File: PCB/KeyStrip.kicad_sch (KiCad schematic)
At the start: 10 parts, among them J2 JST_08

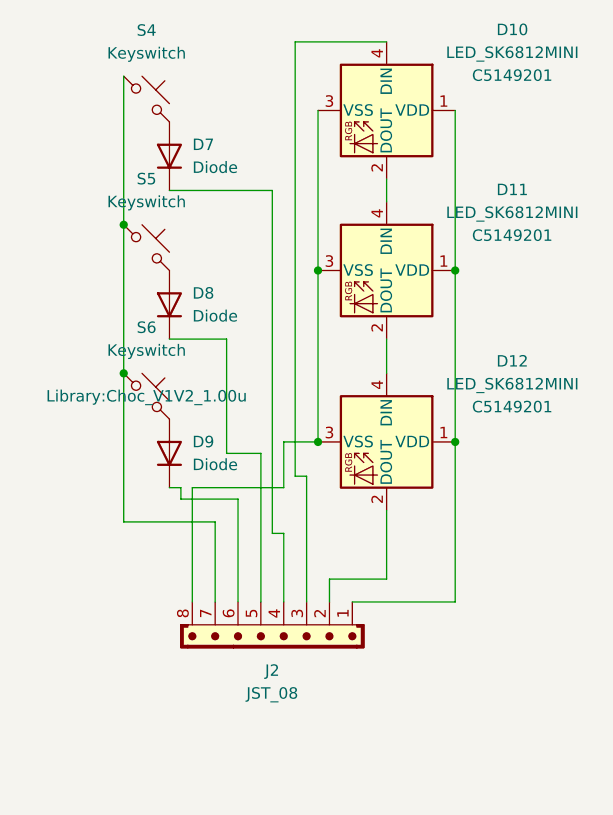
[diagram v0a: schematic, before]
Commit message: I just gotta add screw holes and solo variations now
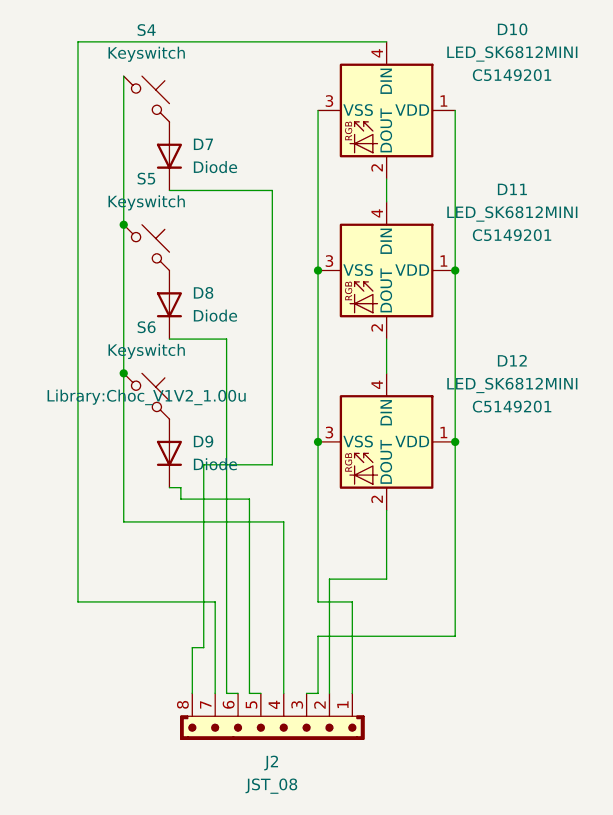
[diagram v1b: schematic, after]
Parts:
- J2: footprint Connector_JST:JST_EH_B8B-EH-A_1x08_P2.50mm_Vertical -> Library:JST_EH_B8B-EH-A_1x08_P2.50mm_Vertical
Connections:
- net at D7.1 (K): now also J2.8; no longer J2.4
- net at S4.1, S5.1, S6.1: now also J2.4; no longer J2.7
- net at D10.1 (VDD), D11.1 (VDD), D12.1 (VDD): now also J2.3; no longer J2.1
- net at D10.4 (DIN): now also J2.7; no longer J2.3
- net at J2.5: now also D9.1 (K); no longer D8.1 (K)
- net at J2.6: now also D8.1 (K); no longer D9.1 (K)
- net at D10.3 (VSS), D11.3 (VSS), D12.3 (VSS): now also J2.1; no longer J2.8
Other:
- moved on the sheet: J2
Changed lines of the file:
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@@
+	)
+	(junction
+		(at 152.4 83.82)
+		(diameter 0)
+		(color 0 0 0 0)
+	)
+	(junction
+		(at 115.57 95.25)
+		(diameter 0)
+		(color 0 0 0 0)
+	)
+	(junction
+		(at 115.57 78.74)
+		(diameter 0)
+		(color 0 0 0 0)
 	)
 	(junction
@@
 	)
 	(junction
-		(at 152.4 83.82)
-		(diameter 0)
-		(color 0 0 0 0)
-	)
-	(junction
-		(at 115.57 95.25)
-		(diameter 0)
-		(color 0 0 0 0)
-	)
-	(junction
-		(at 115.57 78.74)
-		(diameter 0)
-		(color 0 0 0 0)
-	)
-	(junction
 		(at 137.16 102.87)
 		(diameter 0)
@@
 	(wire
 		(pts
+			(xy 125.73 120.65) (xy 125.73 130.81)
+		)
+		(stroke
+			(width 0)
+			(type default)
+		)
+	)
+	(wire
+		(pts
 			(xy 115.57 78.74) (xy 115.57 95.25)
 		)
@@
 	(wire
 		(pts
-			(xy 133.35 102.87) (xy 133.35 107.95)
-		)
-		(stroke
-			(width 0)
-			(type default)
-		)
-	)
-	(wire
-		(pts
-			(xy 130.81 104.14) (xy 130.81 120.65)
+			(xy 124.46 105.41) (xy 124.46 125.73)
+		)
+		(stroke
+			(width 0)
+			(type default)
+		)
+	)
+	(wire
+		(pts
+			(xy 110.49 58.42) (xy 110.49 120.65)
 		)
 		(stroke
@@
 	(wire
 		(pts
-			(xy 128.27 109.22) (xy 128.27 120.65)
-		)
-		(stroke
-			(width 0)
-			(type default)
-		)
-	)
-	(wire
-		(pts
-			(xy 132.08 113.03) (xy 133.35 113.03)
-		)
-		(stroke
-			(width 0)
-			(type default)
-		)
-	)
-	(wire
-		(pts
-			(xy 123.19 107.95) (xy 123.19 120.65)
-		)
-		(stroke
-			(width 0)
-			(type default)
-		)
-	)
-	(wire
-		(pts
-			(xy 135.89 106.68) (xy 135.89 120.65)
-		)
-		(stroke
-			(width 0)
-			(type default)
-		)
-	)
-	(wire
-		(pts
-			(xy 134.62 106.68) (xy 135.89 106.68)
-		)
-		(stroke
-			(width 0)
-			(type default)
-		)
-	)
-	(wire
-		(pts
-			(xy 133.35 107.95) (xy 123.19 107.95)
+			(xy 137.16 124.46) (xy 137.16 130.81)
 		)
 		(stroke
@@
 	(wire
 		(pts
+			(xy 127 130.81) (xy 128.27 130.81)
+		)
+		(stroke
+			(width 0)
+			(type default)
+		)
+	)
+	(wire
+		(pts
 			(xy 115.57 95.25) (xy 115.57 111.76)
 		)
@@
 	(wire
 		(pts
-			(xy 115.57 111.76) (xy 125.73 111.76)
+			(xy 138.43 118.11) (xy 138.43 130.81)
 		)
 		(stroke
@@
 	(wire
 		(pts
-			(xy 138.43 118.11) (xy 138.43 120.65)
-		)
-		(stroke
-			(width 0)
-			(type default)
-		)
-	)
-	(wire
-		(pts
-			(xy 152.4 102.87) (xy 152.4 120.65)
+			(xy 137.16 130.81) (xy 135.89 130.81)
+		)
+		(stroke
+			(width 0)
+			(type default)
+		)
+	)
+	(wire
+		(pts
+			(xy 124.46 125.73) (xy 123.19 125.73)
 		)
 		(stroke
@@
 	(wire
 		(pts
+			(xy 132.08 74.93) (xy 132.08 105.41)
+		)
+		(stroke
+			(width 0)
+			(type default)
+		)
+	)
+	(wire
+		(pts
 			(xy 144.78 91.44) (xy 144.78 95.25)
 		)
@@
 	(wire
 		(pts
-			(xy 137.16 102.87) (xy 133.35 102.87)
-		)
-		(stroke
-			(width 0)
-			(type default)
-		)
-	)
-	(wire
-		(pts
-			(xy 121.92 109.22) (xy 128.27 109.22)
-		)
-		(stroke
-			(width 0)
-			(type default)
-		)
-	)
-	(wire
-		(pts
-			(xy 127 104.14) (xy 130.81 104.14)
+			(xy 121.92 109.22) (xy 129.54 109.22)
 		)
 		(stroke
@@
 	(wire
 		(pts
+			(xy 123.19 125.73) (xy 123.19 130.81)
+		)
+		(stroke
+			(width 0)
+			(type default)
+		)
+	)
+	(wire
+		(pts
+			(xy 110.49 58.42) (xy 144.78 58.42)
+		)
+		(stroke
+			(width 0)
+			(type default)
+		)
+	)
+	(wire
+		(pts
+			(xy 137.16 102.87) (xy 137.16 120.65)
+		)
+		(stroke
+			(width 0)
+			(type default)
+		)
+	)
+	(wire
+		(pts
 			(xy 120.65 91.44) (xy 127 91.44)
 		)
@@
 	(wire
 		(pts
-			(xy 144.78 58.42) (xy 134.62 58.42)
-		)
-		(stroke
-			(width 0)
-			(type default)
-		)
-	)
-	(wire
-		(pts
-			(xy 127 91.44) (xy 127 104.14)
+			(xy 137.16 120.65) (xy 140.97 120.65)
+		)
+		(stroke
+			(width 0)
+			(type default)
+		)
+	)
+	(wire
+		(pts
+			(xy 152.4 124.46) (xy 137.16 124.46)
+		)
+		(stroke
+			(width 0)
+			(type default)
+		)
+	)
+	(wire
+		(pts
+			(xy 152.4 102.87) (xy 152.4 124.46)
+		)
+		(stroke
+			(width 0)
+			(type default)
+		)
+	)
+	(wire
+		(pts
+			(xy 132.08 105.41) (xy 124.46 105.41)
+		)
+		(stroke
+			(width 0)
+			(type default)
+		)
+	)
+	(wire
+		(pts
+			(xy 127 91.44) (xy 127 130.81)
 		)
 		(stroke
@@
 	(wire
 		(pts
-			(xy 152.4 120.65) (xy 140.97 120.65)
-		)
-		(stroke
-			(width 0)
-			(type default)
-		)
-	)
-	(wire
-		(pts
-			(xy 133.35 113.03) (xy 133.35 120.65)
-		)
-		(stroke
-			(width 0)
-			(type default)
-		)
-	)
-	(wire
-		(pts
-			(xy 125.73 111.76) (xy 125.73 120.65)
+			(xy 133.35 111.76) (xy 133.35 130.81)
+		)
+		(stroke
+			(width 0)
+			(type default)
+		)
+	)
+	(wire
+		(pts
+			(xy 115.57 111.76) (xy 133.35 111.76)
+		)
+		(stroke
+			(width 0)
+			(type default)
+		)
+	)
+	(wire
+		(pts
+			(xy 140.97 120.65) (xy 140.97 130.81)
+		)
+		(stroke
+			(width 0)
+			(type default)
+		)
+	)
+	(wire
+		(pts
+			(xy 129.54 109.22) (xy 129.54 130.81)
 		)
 		(stroke
@@
 	(wire
 		(pts
-			(xy 134.62 58.42) (xy 134.62 106.68)
-		)
-		(stroke
-			(width 0)
-			(type default)
-		)
-	)
-	(wire
-		(pts
-			(xy 132.08 74.93) (xy 132.08 113.03)
+			(xy 129.54 130.81) (xy 130.81 130.81)
+		)
+		(stroke
+			(width 0)
+			(type default)
+		)
+	)
+	(wire
+		(pts
+			(xy 110.49 120.65) (xy 125.73 120.65)
 		)
 		(stroke
@@
 	(symbol
 		(lib_id "PCM_SL_Connectors:JST_08")
-		(at 132.08 124.46 270)
+		(at 132.08 134.62 270)
 		(unit 1)
 		(exclude_from_sim no)
@@
 		(fields_autoplaced yes)
 		(property "Reference" "J2"
-			(at 132.08 128.27 90)
+			(at 132.08 138.43 90)
 			(effects
 				(font
@@
 		)
 		(property "Value" "JST_08"
-			(at 132.08 130.81 90)
-			(effects
-				(font
-					(size 1.27 1.27)
-				)
-			)
-		)
-		(property "Footprint" "Connector_JST:JST_EH_B8B-EH-A_1x08_P2.50mm_Vertical"
-			(at 146.05 124.46 0)
+			(at 132.08 140.97 90)
+			(effects
+				(font
+					(size 1.27 1.27)
+				)
+			)
+		)
+		(property "Footprint" "Library:JST_EH_B8B-EH-A_1x08_P2.50mm_Vertical"
+			(at 146.05 134.62 0)
 			(effects
 				(font
@@
 		)
 		(property "Datasheet" ""
-			(at 146.05 124.46 0)
+			(at 146.05 134.62 0)
 			(effects
 				(font
@@
 		)
 		(property "Description" "JST Connector  8 pins"
-			(at 132.08 124.46 0)
-			(effects
-				(font
+			(at 132.08 134.62 0)
+			(effects
+				(font
